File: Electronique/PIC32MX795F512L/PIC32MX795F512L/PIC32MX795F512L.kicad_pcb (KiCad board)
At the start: 2 copper layers, 47.6 x 45.8 mm, 24 parts, among them J101 Conn_02x13_Odd_Even, J102 Conn_02x13_Odd_Even, J103 Conn_02x13_Odd_Even, J104 Conn_02x13_Odd_Even, U101 PIC32MX795F512L, Y101 8Mhz, Y102 Crystal_Small

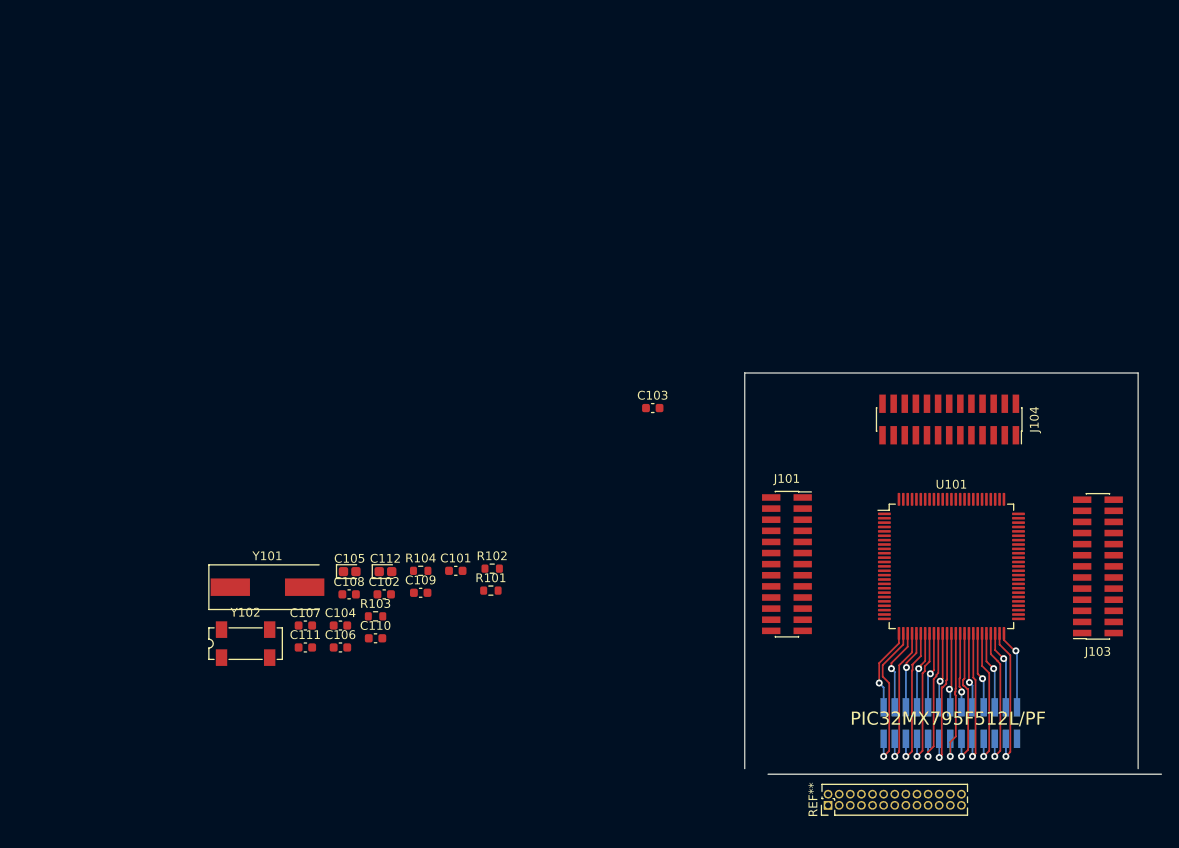
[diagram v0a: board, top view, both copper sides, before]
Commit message: CPU CUBE V2-00
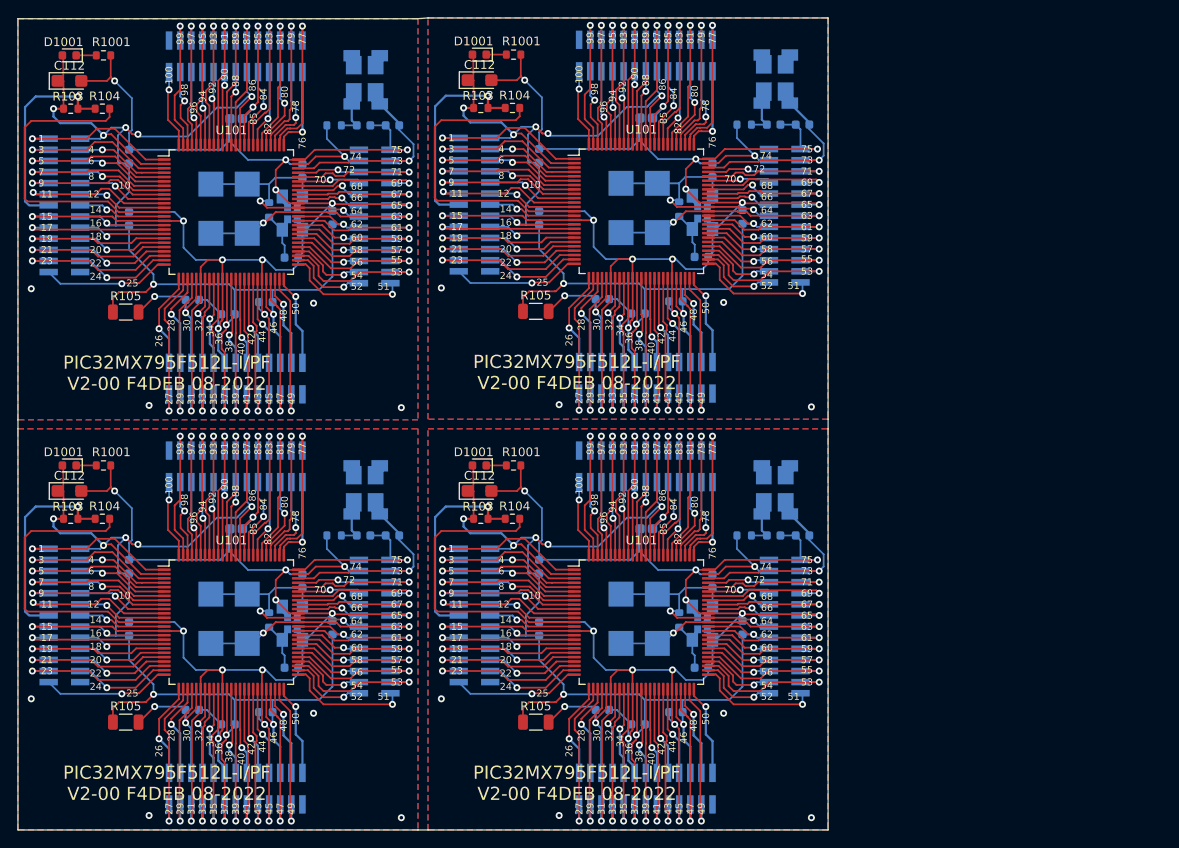
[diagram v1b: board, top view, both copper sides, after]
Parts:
- removed the R101 at (148.8, 100.0)
- removed the REF** at (187.3, 124.6)
- removed Y101: 8Mhz, Crystal:Crystal_SMD_HC49-SD
- removed the Y102 at (120.8, 106.1)
- added C101: 22p, Capacitor_SMD:C_0603_1608Metric, B.Cu at (126.0, 62.0)
- added C101: 22p, Capacitor_SMD:C_0603_1608Metric, B.Cu at (172.8, 108.9)
- added C101: 22p, Capacitor_SMD:C_0603_1608Metric, B.Cu at (126.0, 108.9)
- added C102: 33p, Capacitor_SMD:C_0603_1608Metric, B.Cu at (137.5, 46.9)
- added C102: 33p, Capacitor_SMD:C_0603_1608Metric, B.Cu at (184.4, 93.7)
- added C102: 33p, Capacitor_SMD:C_0603_1608Metric, B.Cu at (137.5, 93.7)
- added C103: 22p, Capacitor_SMD:C_0603_1608Metric, B.Cu at (127.3, 52.1)
- added C103: 22p, Capacitor_SMD:C_0603_1608Metric, B.Cu at (174.1, 99.0)
- added C103: 22p, Capacitor_SMD:C_0603_1608Metric, B.Cu at (127.3, 99.0)
- added C104: 33p, Capacitor_SMD:C_0603_1608Metric, B.Cu at (134.2, 93.7)
- added C104: 33p, Capacitor_SMD:C_0603_1608Metric, B.Cu at (134.2, 46.9)
- added C104: 33p, Capacitor_SMD:C_0603_1608Metric, B.Cu at (181.1, 93.7)
- added C105: 10µ, Capacitor_Tantalum_SMD:CP_EIA-1608-08_AVX-J, B.Cu at (166.5, 93.0)
- added C105: 10µ, Capacitor_Tantalum_SMD:CP_EIA-1608-08_AVX-J, B.Cu at (119.7, 93.0)
- added C105: 10µ, Capacitor_Tantalum_SMD:CP_EIA-1608-08_AVX-J, B.Cu at (119.7, 46.1)
- added C106: 100n, Capacitor_SMD:C_0603_1608Metric, B.Cu at (161.5, 113.7)
- added C106: 100n, Capacitor_SMD:C_0603_1608Metric, B.Cu at (114.7, 113.7)
- added C106: 100n, Capacitor_SMD:C_0603_1608Metric, B.Cu at (114.7, 66.8)
- added C107: 100n, Capacitor_SMD:C_0603_1608Metric, B.Cu at (107.4, 50.4)
- added C107: 100n, Capacitor_SMD:C_0603_1608Metric, B.Cu at (107.4, 97.3)
- added C107: 100n, Capacitor_SMD:C_0603_1608Metric, B.Cu at (154.3, 97.3)
- added C108: 100n, Capacitor_SMD:C_0603_1608Metric, B.Cu at (130.7, 104.3)
- added C108: 100n, Capacitor_SMD:C_0603_1608Metric, B.Cu at (177.5, 104.3)
- added C108: 100n, Capacitor_SMD:C_0603_1608Metric, B.Cu at (130.7, 57.4)
- added C109: 100n, Capacitor_SMD:C_0603_1608Metric, B.Cu at (118.8, 115.3)
- added C109: 100n, Capacitor_SMD:C_0603_1608Metric, B.Cu at (165.6, 115.3)
- added C109: 100n, Capacitor_SMD:C_0603_1608Metric, B.Cu at (118.8, 68.5)
- added C110: 100n, Capacitor_SMD:C_0603_1608Metric, B.Cu at (123.1, 67.1)
- added C110: 100n, Capacitor_SMD:C_0603_1608Metric, B.Cu at (123.1, 113.9)
- added C110: 100n, Capacitor_SMD:C_0603_1608Metric, B.Cu at (169.9, 113.9)
- added C111: 100n, Capacitor_SMD:C_0603_1608Metric, B.Cu at (107.4, 57.6)
- added C111: 100n, Capacitor_SMD:C_0603_1608Metric, B.Cu at (107.4, 104.4)
- added C111: 100n, Capacitor_SMD:C_0603_1608Metric, B.Cu at (154.3, 104.4)
- added C112: 10µ/10V, Capacitor_Tantalum_SMD:CP_EIA-3216-10_Kemet-I, F.Cu at (100.6, 88.7)
- added C112: 10µ/10V, Capacitor_Tantalum_SMD:CP_EIA-3216-10_Kemet-I, F.Cu at (147.5, 88.7)
- added C112: 10µ/10V, Capacitor_Tantalum_SMD:CP_EIA-3216-10_Kemet-I, F.Cu at (100.6, 41.8)
- added D1001: LED, Diode_SMD:D_0603_1608Metric, F.Cu at (100.6, 85.7)
- added D1001: LED, Diode_SMD:D_0603_1608Metric, F.Cu at (147.5, 38.8)
- added D1001: LED, Diode_SMD:D_0603_1608Metric, F.Cu at (100.6, 38.9)
- added D1001: LED, Diode_SMD:D_0603_1608Metric, F.Cu at (147.5, 85.7)
- added J101: Conn_02x13_Odd_Even, Connector_PinSocket_1.27mm:PinSocket_2x13_P1.27mm_Vertical_SMD, B.Cu at (100.1, 56.0)
- added J101: Conn_02x13_Odd_Even, Connector_PinSocket_1.27mm:PinSocket_2x13_P1.27mm_Vertical_SMD, B.Cu at (146.9, 102.9)
- added J101: Conn_02x13_Odd_Even, Connector_PinSocket_1.27mm:PinSocket_2x13_P1.27mm_Vertical_SMD, B.Cu at (100.1, 102.9)
- added J102: Conn_02x13_Odd_Even, Connector_PinSocket_1.27mm:PinSocket_2x13_P1.27mm_Vertical_SMD, B.Cu at (119.6, 75.8)
- added J102: Conn_02x13_Odd_Even, Connector_PinSocket_1.27mm:PinSocket_2x13_P1.27mm_Vertical_SMD, B.Cu at (166.5, 122.7)
- added J102: Conn_02x13_Odd_Even, Connector_PinSocket_1.27mm:PinSocket_2x13_P1.27mm_Vertical_SMD, B.Cu at (119.6, 122.7)
- added J103: Conn_02x13_Odd_Even, Connector_PinSocket_1.27mm:PinSocket_2x13_P1.27mm_Vertical_SMD, B.Cu at (135.5, 104.2)
- added J103: Conn_02x13_Odd_Even, Connector_PinSocket_1.27mm:PinSocket_2x13_P1.27mm_Vertical_SMD, B.Cu at (135.5, 57.3)
- added J103: Conn_02x13_Odd_Even, Connector_PinSocket_1.27mm:PinSocket_2x13_P1.27mm_Vertical_SMD, B.Cu at (182.4, 104.2)
- added J104: Conn_02x13_Odd_Even, Connector_PinSocket_1.27mm:PinSocket_2x13_P1.27mm_Vertical_SMD, B.Cu at (119.6, 85.9)
- added J104: Conn_02x13_Odd_Even, Connector_PinSocket_1.27mm:PinSocket_2x13_P1.27mm_Vertical_SMD, B.Cu at (166.5, 85.9)
- added J104: Conn_02x13_Odd_Even, Connector_PinSocket_1.27mm:PinSocket_2x13_P1.27mm_Vertical_SMD, B.Cu at (119.6, 39.0)
- added R1001: 330, Resistor_SMD:R_0603_1608Metric, F.Cu at (151.4, 85.7)
- added R1001: 330, Resistor_SMD:R_0603_1608Metric, F.Cu at (151.4, 38.8)
- added R1001: 330, Resistor_SMD:R_0603_1608Metric, F.Cu at (104.5, 38.9)
- added R1001: 330, Resistor_SMD:R_0603_1608Metric, F.Cu at (104.5, 85.7)
- added R101: 10M, Resistor_SMD:R_0603_1608Metric, B.Cu at (170.3, 56.4)
- added R101: 10M, Resistor_SMD:R_0603_1608Metric, B.Cu at (170.3, 103.4)
- added R101: 10M, Resistor_SMD:R_0603_1608Metric, B.Cu at (123.4, 56.5)
- added R101: 10M, Resistor_SMD:R_0603_1608Metric, B.Cu at (123.4, 103.4)
- added R102: 2k2, Resistor_SMD:R_0603_1608Metric, B.Cu at (130.9, 93.7)
- added R102: 2k2, Resistor_SMD:R_0603_1608Metric, B.Cu at (130.9, 46.9)
- added R102: 2k2, Resistor_SMD:R_0603_1608Metric, B.Cu at (177.7, 93.7)
- added R103: 10k, Resistor_SMD:R_0603_1608Metric, F.Cu at (100.8, 91.8)
- added R103: 10k, Resistor_SMD:R_0603_1608Metric, F.Cu at (147.6, 91.8)
- added R103: 10k, Resistor_SMD:R_0603_1608Metric, F.Cu at (100.8, 45.0)
- added R104: 470, Resistor_SMD:R_0603_1608Metric, F.Cu at (151.3, 91.8)
- added R104: 470, Resistor_SMD:R_0603_1608Metric, F.Cu at (104.4, 45.0)
- added R104: 470, Resistor_SMD:R_0603_1608Metric, F.Cu at (104.4, 91.8)
- added R105: 0, Resistor_SMD:R_1206_3216Metric, F.Cu at (153.9, 68.1)
- added R105: 0, Resistor_SMD:R_1206_3216Metric, F.Cu at (153.9, 115.1)
- added R105: 0, Resistor_SMD:R_1206_3216Metric, F.Cu at (107.1, 68.2)
- added R105: 0, Resistor_SMD:R_1206_3216Metric, F.Cu at (107.1, 115.1)
- added REF**: Crystal_SMD_SeikoEpson_MC306-4Pin_8.0x3.2mm_HandSoldering, Crystal:Crystal_SMD_SeikoEpson_MC306-4Pin_8.0x3.2mm_HandSoldering, B.Cu at (118.9, 56.4)
- added REF**: Crystal_SMD_SeikoEpson_MC306-4Pin_8.0x3.2mm_HandSoldering, Crystal:Crystal_SMD_SeikoEpson_MC306-4Pin_8.0x3.2mm_HandSoldering, B.Cu at (118.9, 103.3)
- added REF**: Crystal_SMD_SeikoEpson_FA238V-4Pin_3.2x2.5mm_HandSoldering, Crystal:Crystal_SMD_SeikoEpson_FA238V-4Pin_3.2x2.5mm_HandSoldering, B.Cu at (134.4, 88.4)
- added REF**: Crystal_SMD_SeikoEpson_FA238V-4Pin_3.2x2.5mm_HandSoldering, Crystal:Crystal_SMD_SeikoEpson_FA238V-4Pin_3.2x2.5mm_HandSoldering, B.Cu at (181.2, 88.4)
- added REF**: Crystal_SMD_SeikoEpson_FA238V-4Pin_3.2x2.5mm_HandSoldering, Crystal:Crystal_SMD_SeikoEpson_FA238V-4Pin_3.2x2.5mm_HandSoldering, B.Cu at (181.2, 41.5)
- added REF**: Crystal_SMD_SeikoEpson_FA238V-4Pin_3.2x2.5mm_HandSoldering, Crystal:Crystal_SMD_SeikoEpson_FA238V-4Pin_3.2x2.5mm_HandSoldering, B.Cu at (134.4, 41.5)
- added REF**: Crystal_SMD_2016-4Pin_2.0x1.6mm, Crystal:Crystal_SMD_2016-4Pin_2.0x1.6mm, B.Cu at (126.1, 103.8)
- added REF**: Crystal_SMD_2016-4Pin_2.0x1.6mm, Crystal:Crystal_SMD_2016-4Pin_2.0x1.6mm, B.Cu at (173.0, 103.8)
- added REF**: Crystal_SMD_2016-4Pin_2.0x1.6mm, Crystal:Crystal_SMD_2016-4Pin_2.0x1.6mm, B.Cu at (126.1, 56.9)
- added REF**: Crystal_SMD_SeikoEpson_MC306-4Pin_8.0x3.2mm_HandSoldering, Crystal:Crystal_SMD_SeikoEpson_MC306-4Pin_8.0x3.2mm_HandSoldering, B.Cu at (165.7, 103.3)
- added REF**: Crystal_SMD_SeikoEpson_MC306-4Pin_8.0x3.2mm_HandSoldering, Crystal:Crystal_SMD_SeikoEpson_MC306-4Pin_8.0x3.2mm_HandSoldering, B.Cu at (165.7, 56.3)
- added REF**: Crystal_SMD_2016-4Pin_2.0x1.6mm, Crystal:Crystal_SMD_2016-4Pin_2.0x1.6mm, B.Cu at (173.0, 56.8)
- added U101: PIC32MX795F512L, Package_QFP:TQFP-100_14x14mm_P0.5mm, F.Cu at (119.1, 103.7)
- added U101: PIC32MX795F512L, Package_QFP:TQFP-100_14x14mm_P0.5mm, F.Cu at (119.1, 56.8)
- added U101: PIC32MX795F512L, Package_QFP:TQFP-100_14x14mm_P0.5mm, F.Cu at (166.0, 103.7)
- added Y1001: 8Mhz, Crystal:Crystal_SMD_Abracon_ABM3C-4Pin_5.0x3.2mm, B.Cu at (126.1, 56.9)
- added Y1001: 8Mhz, Crystal:Crystal_SMD_Abracon_ABM3C-4Pin_5.0x3.2mm, B.Cu at (126.1, 103.8)
- added Y1001: 8Mhz, Crystal:Crystal_SMD_Abracon_ABM3C-4Pin_5.0x3.2mm, B.Cu at (173.0, 103.8)
- added Y1001: 8Mhz, Crystal:Crystal_SMD_Abracon_ABM3C-4Pin_5.0x3.2mm, B.Cu at (173.0, 56.8)
- added Y102: Crystal_Small, Crystal:Crystal_SMD_SeikoEpson_MC306-4Pin_8.0x3.2mm, B.Cu at (134.5, 41.7)
- added Y102: Crystal_Small, Crystal:Crystal_SMD_SeikoEpson_MC306-4Pin_8.0x3.2mm, B.Cu at (134.5, 88.5)
- added Y102: Crystal_Small, Crystal:Crystal_SMD_SeikoEpson_MC306-4Pin_8.0x3.2mm, B.Cu at (181.4, 88.5)
- added Y102: Crystal_Small, Crystal:Crystal_SMD_SeikoEpson_MC306-4Pin_8.0x3.2mm, B.Cu at (181.4, 41.6)
- C101, C102, C103, C104, C105, C106, C107, C108, C109, C110, C111, J101, J103, J104, R102: moved to B.Cu
- C112: footprint Capacitor_Tantalum_SMD:CP_EIA-1608-08_AVX-J -> Capacitor_Tantalum_SMD:CP_EIA-3216-10_Kemet-I
- moved C104 75.7 mm to (181.1, 46.8)
- moved C102 71.9 mm to (184.4, 46.8), turned to 180 degrees
- moved C108 62.3 mm to (177.5, 57.3), turned to 90 degrees
- moved C105 61.9 mm to (166.5, 46.0), turned to 180 degrees
- moved C107 60.0 mm to (154.3, 50.4), turned to 90 degrees
- moved R103 59.3 mm to (147.6, 44.9)
- moved R102 58.3 mm to (177.7, 46.8)
- moved C112 57.2 mm to (147.5, 41.7)
- moved C111 55.9 mm to (154.3, 57.5), turned to 90 degrees
- moved J101 54.4 mm to (146.9, 55.9), turned to 180 degrees
- moved J104 54.1 mm to (166.5, 38.9), turned to 90 degrees
- moved R104 53.9 mm to (151.3, 44.9)
- moved U101 53.9 mm to (166.0, 56.7)
- moved J103 53.7 mm to (182.4, 57.2), turned to 0 degrees
- moved J102 52.6 mm to (166.5, 75.7)
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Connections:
- C101 pad 1: Net-(C101-Pad1) -> /63
- C102 pad 1: Net-(C102-Pad1) -> /73
- C103 pad 1: Net-(C103-Pad1) -> /64
- C105 pad 1: Net-(C105-Pad1) -> /85
- R102 pad 1: Net-(R102-Pad1) -> /74
- U101 pad 63: Net-(C101-Pad1) -> /63
- U101 pad 64: Net-(C103-Pad1) -> /64
- U101 pad 73: Net-(C102-Pad1) -> /73
- U101 pad 74: Net-(R102-Pad1) -> /74
- U101 pad 85: Net-(C105-Pad1) -> /85
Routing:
- net GND: track 42.1 -> 794.4 mm, vias 3 -> 72
- net +3V3: track 25.6 -> 666.2 mm, vias 2 -> 44
- net Net-(R104-Pad2): track 0.00 -> 143.5 mm
- net /63: track 0.00 -> 128.4 mm, vias 0 -> 8
- net /64: track 0.00 -> 116.9 mm, vias 0 -> 8
- net /13: track 0.00 -> 97.9 mm, vias 0 -> 4
- net /73: track 0.00 -> 92.9 mm, vias 0 -> 4
- net /1: track 0.00 -> 75.5 mm, vias 0 -> 4
- net /3: track 0.00 -> 74.2 mm, vias 0 -> 4
- net /5: track 0.00 -> 72.5 mm, vias 0 -> 4
- net /23: track 0.00 -> 72.1 mm, vias 0 -> 4
- net /11: track 0.00 -> 71.5 mm, vias 0 -> 4
- net /9: track 0.00 -> 71.1 mm, vias 0 -> 4
- net /7: track 0.00 -> 71.0 mm, vias 0 -> 4
- net /85: track 0.00 -> 70.8 mm, vias 0 -> 8
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- added copper zone on B.Cu, net GND
- added copper zone on F.Cu, net GND
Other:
- board size 47.6 x 45.8 mm -> 92.6 x 92.8 mm
- board text added: "1"
- board text added: "10"
- board text added: "100"
- board text added: "11"
- board text added: "12"
- board text added: "14"
- board text added: "15"
- board text added: "16"
- board text added: "17"
- board text added: "18"
- board text added: "19"
- board text added: "20"
- board text added: "21"
- board text added: "22"
- board text added: "23"
- board text added: "24"
- board text added: "25"
- board text added: "26"
- board text added: "27"
- board text added: "28"
- board text added: "29"
- board text added: "3"
- board text added: "30"
- board text added: "31"
- board text added: "32"
- board text added: "33"
- board text added: "34"
- board text added: "35"
- board text added: "36"
- board text added: "37"
- board text added: "38"
- board text added: "39"
- board text added: "4"
- board text added: "40"
- board text added: "41"
- board text added: "42"
- board text added: "43"
- board text added: "44"
- board text added: "45"
- board text added: "46"
- board text added: "47"
- board text added: "48"
- board text added: "49"
- board text added: "5"
- board text added: "50"
- board text added: "51"
- board text added: "52"
- board text added: "53"
- board text added: "54"
- board text added: "55"
- board text added: "56"
- board text added: "57"
- board text added: "58"
- board text added: "59"
- board text added: "6"
- board text added: "60"
- board text added: "61"
- board text added: "62"
- board text added: "63"
- board text added: "64"
- board text added: "65"
- board text added: "66"
- board text added: "67"
- board text added: "68"
- board text added: "69"
- board text added: "7"
- board text added: "70"
- board text added: "71"
- board text added: "72"
- board text added: "73"
- board text added: "74"
- board text added: "75"
- board text added: "76"
- board text added: "77"
- board text added: "78"
- board text added: "79"
- board text added: "8"
- board text added: "80"
- board text added: "81"
- board text added: "82"
- board text added: "83"
- board text added: "84"
- board text added: "85"
- board text added: "86"
- board text added: "87"
- board text added: "88"
- board text added: "89"
- board text added: "9"
- board text added: "90"
- board text added: "91"
- board text added: "92"
- board text added: "93"
- board text added: "94"
- board text added: "95"
- board text added: "96"
- board text added: "97"
- board text added: "98"
- board text added: "99"
- board text added: "PIC32MX795F512L-I/PF V2-00 F4DEB 08-2022"
- board text removed: "PIC32MX795F512L/PF"
